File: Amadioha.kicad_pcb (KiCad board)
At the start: 4 copper layers, 74 x 49.9 mm, 66 parts, among them IC1 ACS37800KMACTR-030B3-I2C, J1 691137710002, J2 SW_Debug, J3 691137710002, K1 G6DN-1A-SL_DC5, Q1 BSS138, Q2 BSS138, Q3 BSS138, SW1 PTS815, SW2 PTS815, U1 STM32WB55CGU6, U2 NCP1117-3.3_SOT223, Y1 32MHz, Y2 32K768

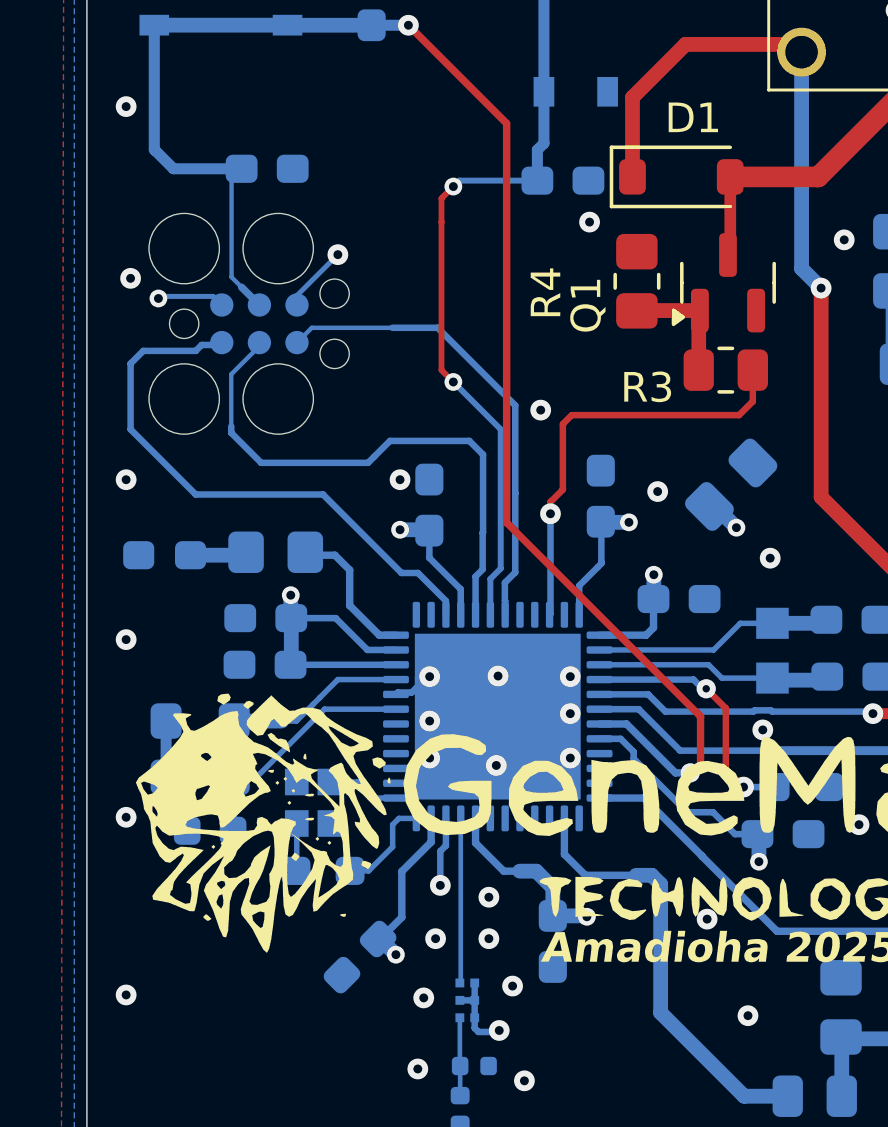
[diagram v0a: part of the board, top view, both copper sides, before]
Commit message: 1/7/2026
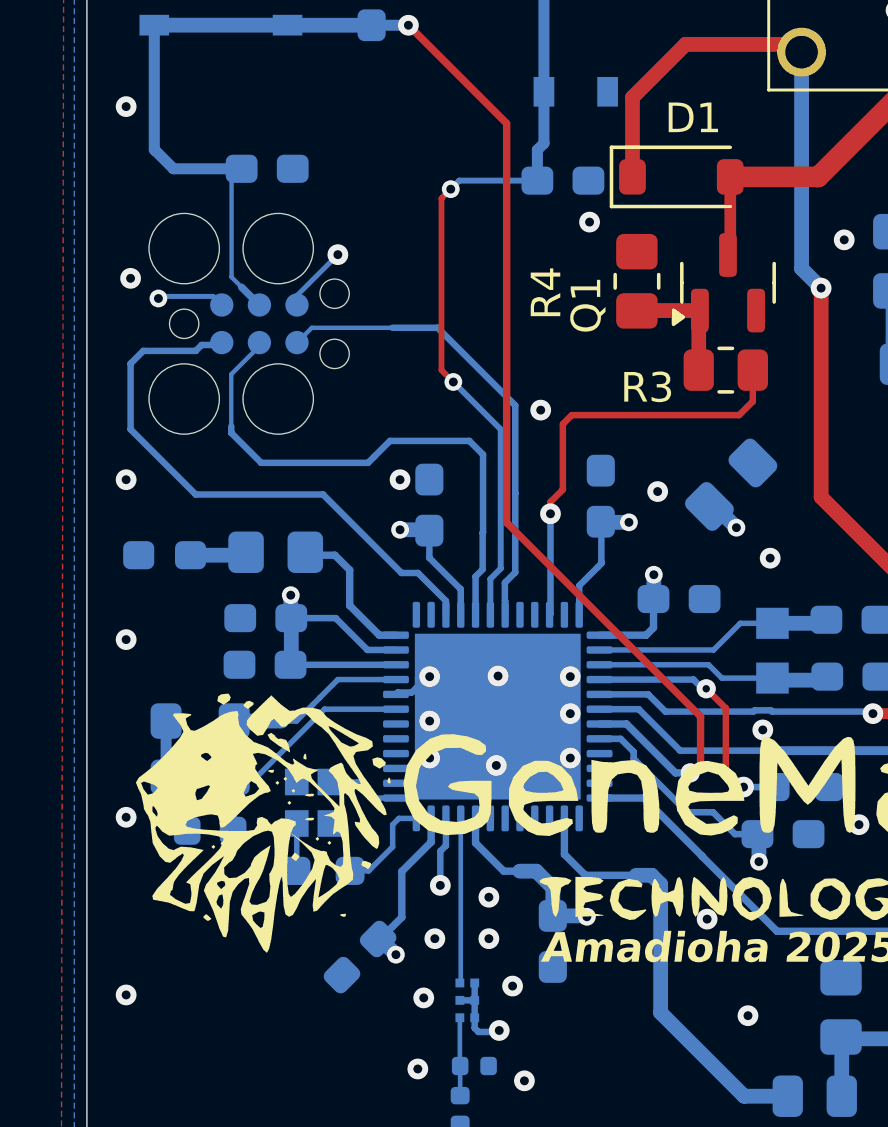
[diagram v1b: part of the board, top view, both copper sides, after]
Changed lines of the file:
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@@
 	(generator_version "9.0")
 	(general
-		(thickness 1.5842)
+		(thickness 1.6002)
 		(legacy_teardrops no)
 	)
@@
 			(layer "F.Mask"
 				(type "Top Solder Mask")
-				(thickness 0.01)
+				(thickness 0.02)
 			)
 			(layer "F.Cu"
@@
 			(layer "B.Mask"
 				(type "Bottom Solder Mask")
-				(thickness 0.01)
+				(thickness 0.016)
 			)
 			(layer "B.Paste"
@@
 		(layer "F.Cu")
 		(pts
-			(xy 151.4 109.1375) (xy 152 58.294312)
+			(xy 89.725 95.175) (xy 89.975 95.225)
 		)
-		(height 7.6)
-		(orientation 1)
+		(height 18.375)
+		(orientation 0)
 		(format
 			(prefix "")
@@
 			(keep_text_aligned yes)
 		)
-		(gr_text "50.8432 mm"
-			(at 157.2 83.715906 90)
-			(layer "F.Cu")
-			(effects
-				(font
-					(size 1.5 1.5)
-					(thickness 0.3)
-				)
-			)
-		)
-	)
-	(dimension
-		(type orthogonal)
-		(layer "F.Cu")
-		(pts
-			(xy 122.825 109.9375) (xy 122.825 58.3375)
-		)
-		(height 44)
-		(orientation 1)
-		(format
-			(prefix "")
-			(suffix "")
-			(units 3)
-			(units_format 1)
-			(precision 4)
-		)
-		(style
-			(thickness 0.2)
-			(arrow_length 1.27)
-			(text_position_mode 0)
-			(arrow_direction outward)
-			(extension_height 0.58642)
-			(extension_offset 0.5)
-			(keep_text_aligned yes)
-		)
-		(gr_text "51.6000 mm"
-			(at 165.025 84.1375 90)
+		(gr_text "0.2500 mm"
+			(at 89.85 111.75 0)
 			(layer "F.Cu")
 			(effects
@@
 	)
 	(via
-		(at 89.2 94.6)
+		(at 89.175 94.6)
 		(size 0.7)
 		(drill 0.3)
@@
 	)
 	(segment
-		(start 89.4 70.4)
-		(end 89.4 69.6)
-		(width 0.2)
-		(layer "F.Cu")
-		(net 47)
-	)
-	(segment
-		(start 89.4 75.4)
-		(end 89.4 70.4)
+		(start 89.4 69.6)
+		(end 89.4 75.4)
 		(width 0.2)
 		(layer "F.Cu")
@@
 	)
 	(segment
-		(start 89.4 69.6)
-		(end 89.8 69.2)
+		(start 89.7125 69.2875)
+		(end 89.4 69.6)
 		(width 0.2)
 		(layer "F.Cu")
@@
 	)
 	(segment
-		(start 89.8 75.8)
-		(end 89.4 75.4)
+		(start 89.4 75.4)
+		(end 89.8 75.8)
 		(width 0.2)
 		(layer "F.Cu")
@@
 	)
 	(via
-		(at 89.8 69.2)
+		(at 89.7125 69.2875)
 		(size 0.6)
 		(drill 0.3)
@@
 	)
 	(segment
-		(start 90 69)
-		(end 92.6375 69)
-		(width 0.2)
-		(layer "B.Cu")
-		(net 47)
-	)
-	(segment
 		(start 92.86 67.74)
 		(end 92.86 66)
@@
 	)
 	(segment
-		(start 89.8 69.2)
-		(end 90 69)
-		(width 0.2)
-		(layer "B.Cu")
-		(net 47)
-	)
-	(segment
 		(start 92.6375 67.9625)
 		(end 92.86 67.74)
@@
 		(width 0.2)
 		(layer "B.Cu")
+		(net 47)
+	)
+	(segment
+		(start 89.7125 69.2875)
+		(end 90 69)
+		(width 0.2)
+		(layer "B.Cu")
+		(net 47)
+	)
+	(segment
+		(start 90 69)
+		(end 92.6375 69)
+		(width 0.2)
+		(layer "B.Cu")
